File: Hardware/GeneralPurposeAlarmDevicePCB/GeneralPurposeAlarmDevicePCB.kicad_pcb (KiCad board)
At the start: 2 copper layers, 137.2 x 83.8 mm, 131 parts, among them J101 Barrel_Jack_Switch_SMT, J102 0.100_2Pin, J103 0.100_2Pin, J105 S04B-XASK-1(LF)(SN), J401 RJ12_6P6C_HORZ, J501 USB_B_Micro_Local, J601 22-23-2021, J602 22-23-2021, Q201 MMBT2222A-7-F, Q202 MMBT2222A-7-F, Q203 MMBT2222A-7-F, Q204 MMBT2222A-7-F, Q205 MMBT2222A-7-F, Q301 BSS138, Q601 MMBT2222A-7-F, Q602 MMBT2907ALT1G, T1 JLC_ToolingHole_0576mm, T2 JLC_ToolingHole_0576mm, T3 JLC_ToolingHole_0576mm, U101 LM7805_TO220, U102 PI_ATMEGA328P-AU-InOrder, U301 PCF8574AT, U302 LCD_20x4_Character-GPAD_SCH_L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, U501 CH340E

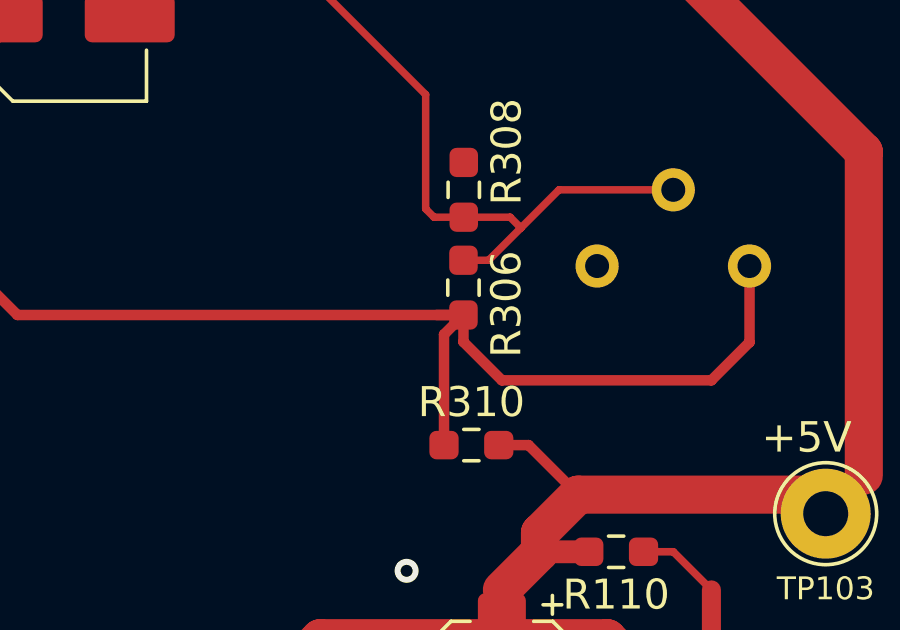
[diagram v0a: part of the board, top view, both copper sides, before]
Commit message: Delete stray track.
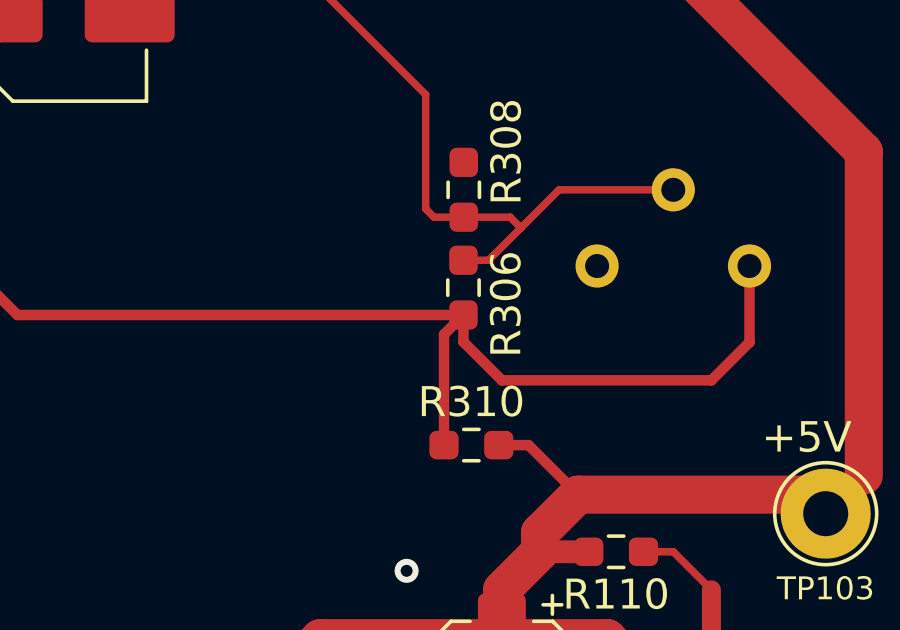
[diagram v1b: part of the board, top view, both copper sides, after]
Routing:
- net /LCD And I2C Interface/Vcc_LCD: track 120.3 -> 119.4 mm
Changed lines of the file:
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@@
   (segment (start 158.75 30.48) (end 163.195 30.48) (width 1.27) (layer "F.Cu") (net 67))
   (segment (start 162.900004 33.02) (end 161.925 33.995004) (width 1.27) (layer "F.Cu") (net 67))
-  (segment (start 177.5275 42.9075) (end 178.425 42.9075) (width 0.35) (layer "F.Cu") (net 67))
   (segment (start 135.89 34.925) (end 138.0725 37.1075) (width 0.35) (layer "F.Cu") (net 67))
   (segment (start 164.2375 27.94) (end 164.2375 27.220002) (width 0.35) (layer "F.Cu") (net 67))
